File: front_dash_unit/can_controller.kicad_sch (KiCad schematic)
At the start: 11 parts, among them U8 TJA1050T_CM_118, U9 MCP2515-xST, Y5 20MHz

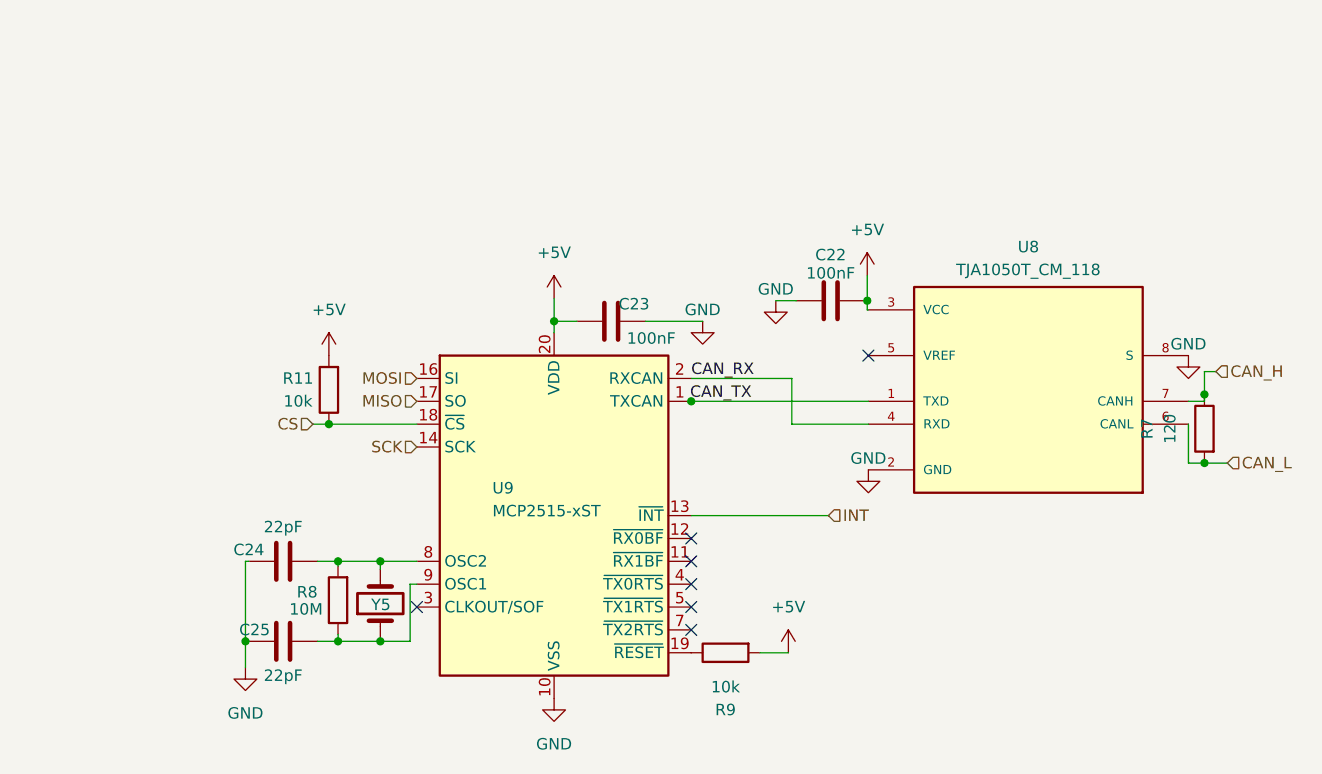
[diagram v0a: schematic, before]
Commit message: front dash review
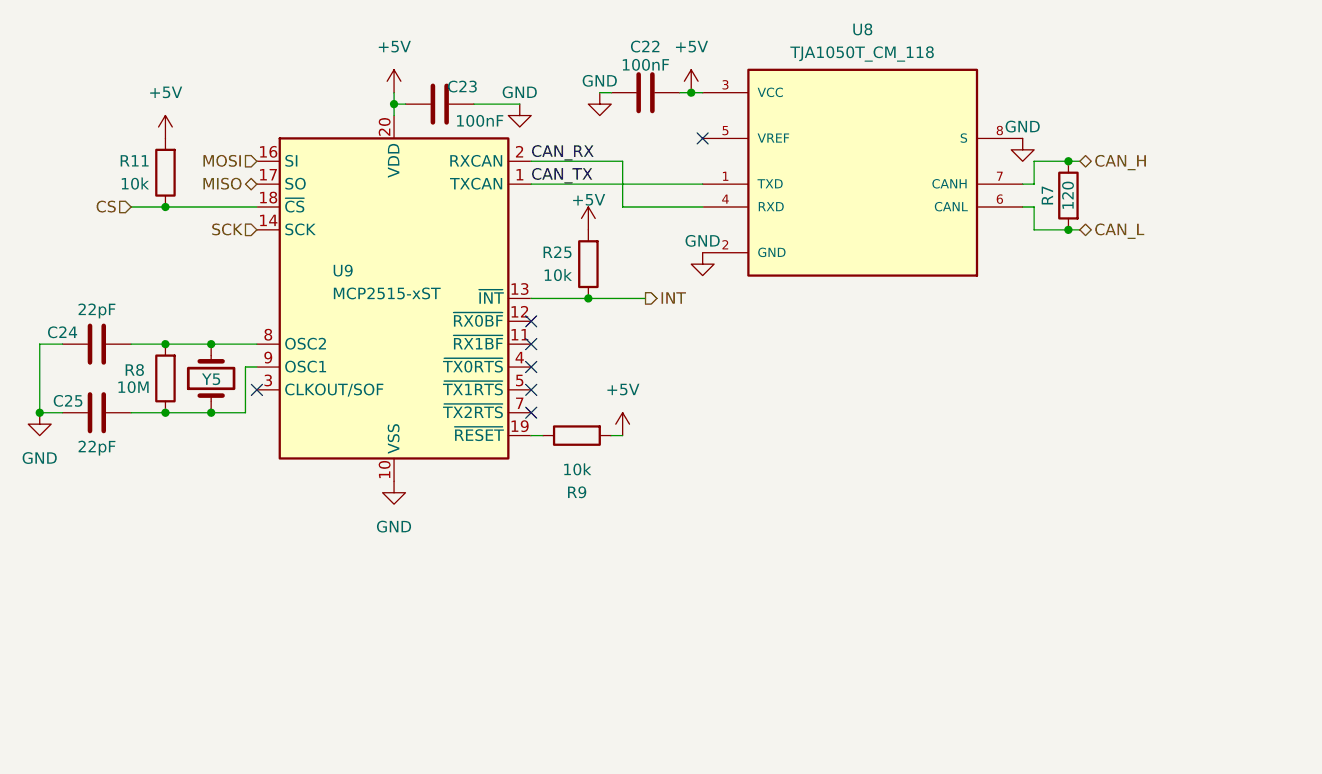
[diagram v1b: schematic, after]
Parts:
- added R25: 10k, Better_Handsolder:R_0805_2012Metric_Pad1.20x1.40mm_HandSolder_L, symbol Device:R
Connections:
- net +5V: now also R25.2
- net INT: now also R25.1
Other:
- moved on the sheet: C22, C23, C24, C25, R11, R7, R8, R9, U8, U9, Y5

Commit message: dash update
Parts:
- C22, C23, C24, C25: footprint Better_Handsolder:C_0805_2012Metric_Pad1.18x1.45mm_HandSolder_L -> RMC_Capacitor:C_0805_2012Metric_Pad1.18x1.45mm_HandSolder_L
- R11, R25, R7, R8, R9: footprint Better_Handsolder:R_0805_2012Metric_Pad1.20x1.40mm_HandSolder_L -> RMC_Resistor:R_0805_2012Metric_Pad1.20x1.40mm_HandSolder_L
- U8: footprint TJA1050T_CM_118:SOIC127P600X175-8N -> RMC_SO:SOIC-8_3.9x4.9mm_P1.27mm_RMC_Handsolder
- U9: footprint Package_SO:SSOP-20_4.4x6.5mm_P0.65mm -> RMC_SO:TSSOP-20_4.4x6.5mm_P0.65mm
- Y5: footprint Better_Handsolder:Crystal_HC49-U_Vertical_W_SMD -> Crystal:Crystal_HC49-U_Vertical
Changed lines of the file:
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@@
 			)
 		)
-		(property "Footprint" "Better_Handsolder:R_0805_2012Metric_Pad1.20x1.40mm_HandSolder_L"
+		(property "Footprint" "RMC_Resistor:R_0805_2012Metric_Pad1.20x1.40mm_HandSolder_L"
 			(at 86.868 59.69 90)
 			(hide yes)
@@
 			)
 		)
-		(property "Footprint" "Package_SO:SSOP-20_4.4x6.5mm_P0.65mm"
+		(property "Footprint" "RMC_SO:TSSOP-20_4.4x6.5mm_P0.65mm"
 			(at 110.49 96.52 0)
 			(hide yes)
@@
 			)
 		)
-		(property "Footprint" "Better_Handsolder:R_0805_2012Metric_Pad1.20x1.40mm_HandSolder_L"
+		(property "Footprint" "RMC_Resistor:R_0805_2012Metric_Pad1.20x1.40mm_HandSolder_L"
 			(at 187.198 62.23 90)
 			(hide yes)
@@
 			)
 		)
-		(property "Footprint" "Better_Handsolder:C_0805_2012Metric_Pad1.18x1.45mm_HandSolder_L"
+		(property "Footprint" "RMC_Capacitor:C_0805_2012Metric_Pad1.18x1.45mm_HandSolder_L"
 			(at 81.28 87.3252 0)
 			(hide yes)
@@
 			)
 		)
-		(property "Footprint" "Better_Handsolder:R_0805_2012Metric_Pad1.20x1.40mm_HandSolder_L"
+		(property "Footprint" "RMC_Resistor:R_0805_2012Metric_Pad1.20x1.40mm_HandSolder_L"
 			(at 133.858 69.85 90)
 			(hide yes)
@@
 			)
 		)
-		(property "Footprint" "Better_Handsolder:C_0805_2012Metric_Pad1.18x1.45mm_HandSolder_L"
+		(property "Footprint" "RMC_Capacitor:C_0805_2012Metric_Pad1.18x1.45mm_HandSolder_L"
 			(at 142.24 51.7652 0)
 			(hide yes)
@@
 			)
 		)
-		(property "Footprint" "Better_Handsolder:C_0805_2012Metric_Pad1.18x1.45mm_HandSolder_L"
+		(property "Footprint" "RMC_Capacitor:C_0805_2012Metric_Pad1.18x1.45mm_HandSolder_L"
 			(at 111.76 53.0352 0)
 			(hide yes)
@@
 			)
 		)
-		(property "Footprint" "Better_Handsolder:Crystal_HC49-U_Vertical_W_SMD"
+		(property "Footprint" "Crystal:Crystal_HC49-U_Vertical"
 			(at 90.17 82.55 0)
 			(hide yes)
@@
 			)
 		)
-		(property "Footprint" "Better_Handsolder:C_0805_2012Metric_Pad1.18x1.45mm_HandSolder_L"
+		(property "Footprint" "RMC_Capacitor:C_0805_2012Metric_Pad1.18x1.45mm_HandSolder_L"
 			(at 81.28 77.7748 0)
 			(hide yes)
@@
 			)
 		)
-		(property "Footprint" "Better_Handsolder:R_0805_2012Metric_Pad1.20x1.40mm_HandSolder_L"
+		(property "Footprint" "RMC_Resistor:R_0805_2012Metric_Pad1.20x1.40mm_HandSolder_L"
 			(at 86.868 82.55 90)
 			(hide yes)
@@
 			)
 		)
-		(property "Footprint" "Better_Handsolder:R_0805_2012Metric_Pad1.20x1.40mm_HandSolder_L"
+		(property "Footprint" "RMC_Resistor:R_0805_2012Metric_Pad1.20x1.40mm_HandSolder_L"
 			(at 130.81 87.122 90)
 			(hide yes)
@@
 			)
 		)
-		(property "Footprint" "TJA1050T_CM_118:SOIC127P600X175-8N"
+		(property "Footprint" "RMC_SO:SOIC-8_3.9x4.9mm_P1.27mm_RMC_Handsolder"
 			(at 162.56 58.42 0)
 			(hide yes)
